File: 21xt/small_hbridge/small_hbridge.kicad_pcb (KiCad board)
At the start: 2 copper layers, 70.6 x 47 mm, 19 parts, among them J1 Screw_Terminal_01x02, J2 Screw_Terminal_01x02, J4 Conn_01x10, U1 VNH5019ATR-E, U2 STD3NK100Z

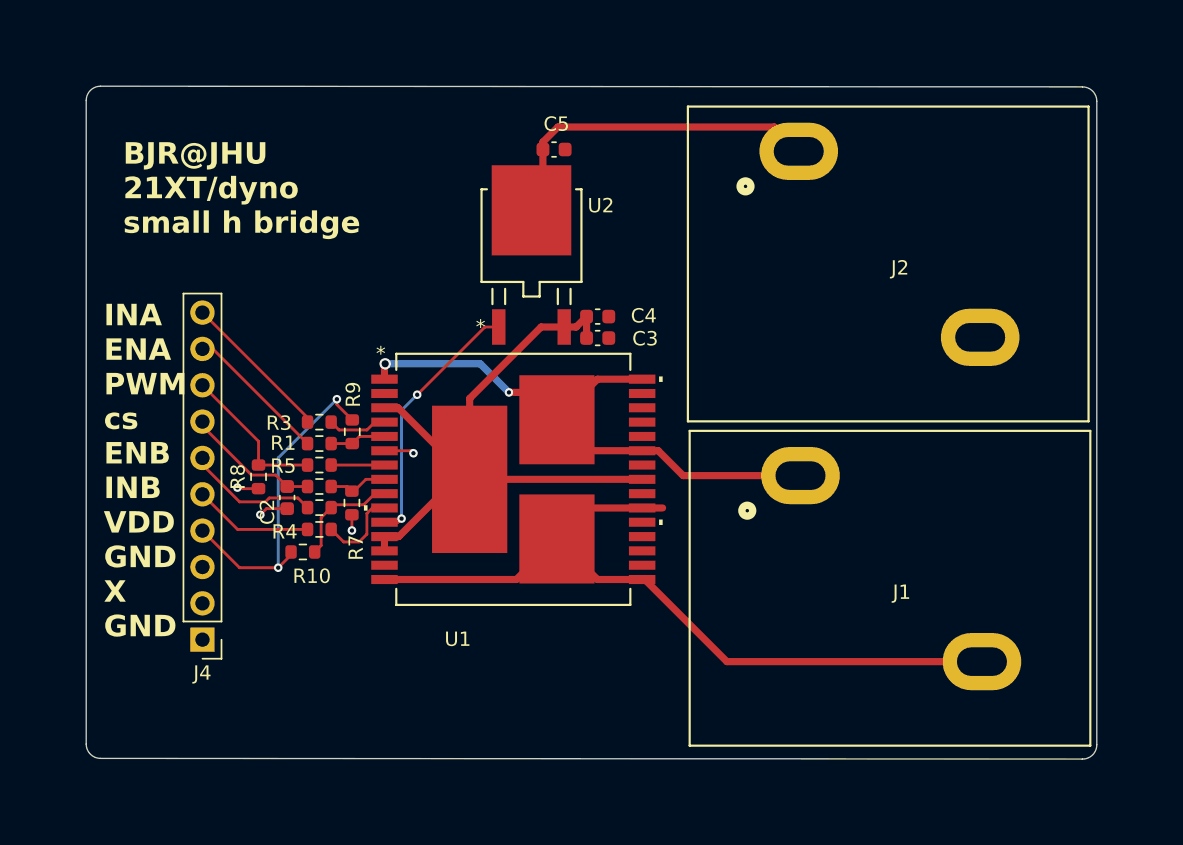
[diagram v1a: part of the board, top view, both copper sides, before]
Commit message: aaaaa
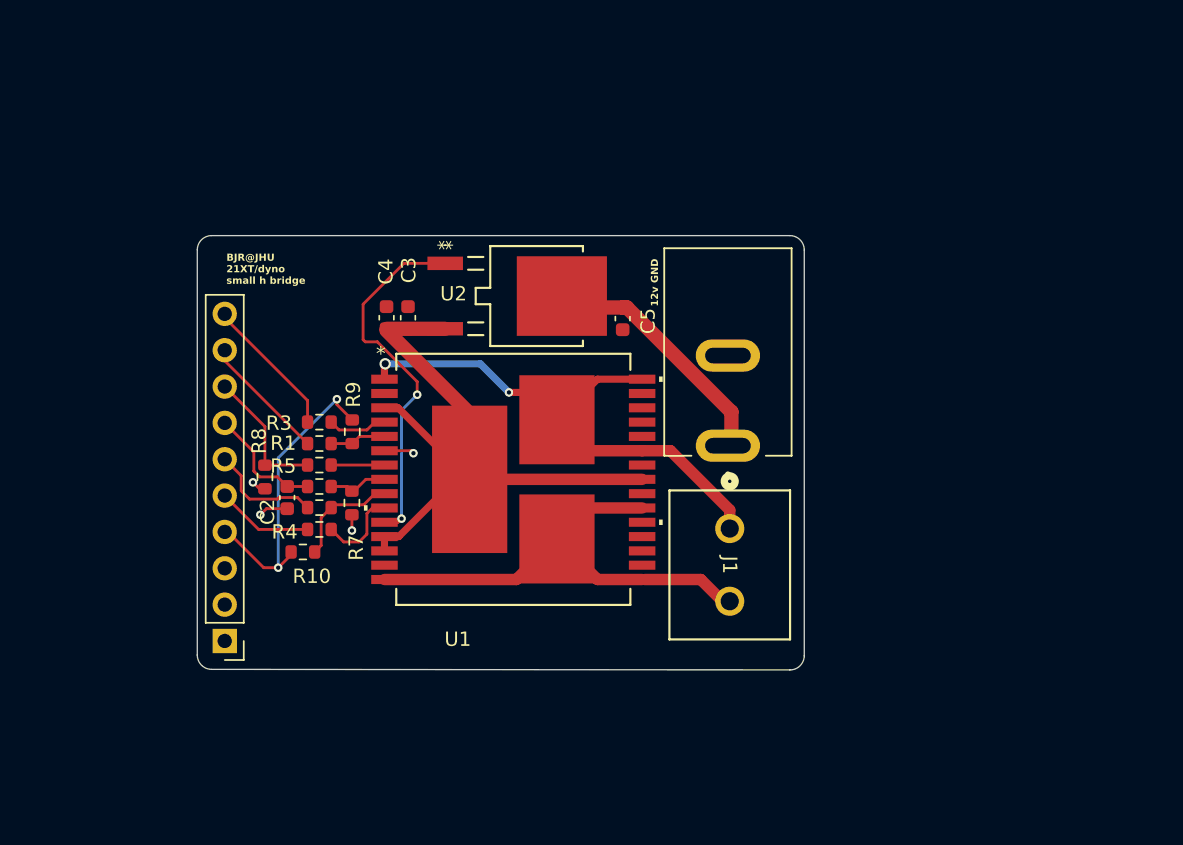
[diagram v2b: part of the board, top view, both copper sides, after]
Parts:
- removed J2: Screw_Terminal_01x02, dynoinst_fp:CONN_4DB-P108-02_TEC
- added J3: Barrel_Jack, dynoinst_fp:CUI_PJ-037A, F.Cu at (190.2, 87.2)
- J1: footprint dynoinst_fp:CONN_4DB-P108-02_TEC -> dynoinst_fp:282837-2_TYC
- moved C4 14.8 mm to (166.4, 78.3), turned to -90 degrees
- moved C3 13.3 mm to (167.9, 78.3), turned to -90 degrees
- moved C5 12.8 mm to (182.9, 78.3), turned to 90 degrees
- moved J1 7.21 mm to (190.4, 93.0), turned to -90 degrees
- moved U2 4.24 mm to (176.9, 76.7), turned to -90 degrees
- moved J4 1.56 mm to (155.1, 100.8)
- moved R8 0.45 mm to (157.9, 89.4)
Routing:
- net OUTB: track 54.8 -> 34.0 mm
- net 12v: track 26.3 -> 18.0 mm
- net Net-(U1-CP): track 18.1 -> 25.7 mm
- net OUTA: track 40.5 -> 37.8 mm
- net INB: track 8.36 -> 6.77 mm
- net VDD: track 23.2 -> 21.6 mm
- net ENB: track 9.29 -> 7.90 mm
- net ENA: track 10.1 -> 8.92 mm
- net CURRSNS: track 9.40 -> 8.41 mm
- net PWM: track 10.6 -> 9.76 mm
- net 12v': track 46.4 -> 45.7 mm
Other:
- board size 70.6 x 47 mm -> 42.4 x 30.4 mm
- board text added: "12v GND"
